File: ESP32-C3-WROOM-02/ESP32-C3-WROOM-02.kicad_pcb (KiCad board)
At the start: 2 copper layers, 25.4 x 38.1 mm, 22 parts, among them J1 ESP32-C3-DEVKITC-02-J1, J2 ESP32-C3-DEVKITC-02-J2, J3 ESPProg-UART, J4 USB2.0_C, SW1 SW_Push, SW2 SW_Push, U1 AMS1117-3.3, U2 ESP32-C3-WROOM-02

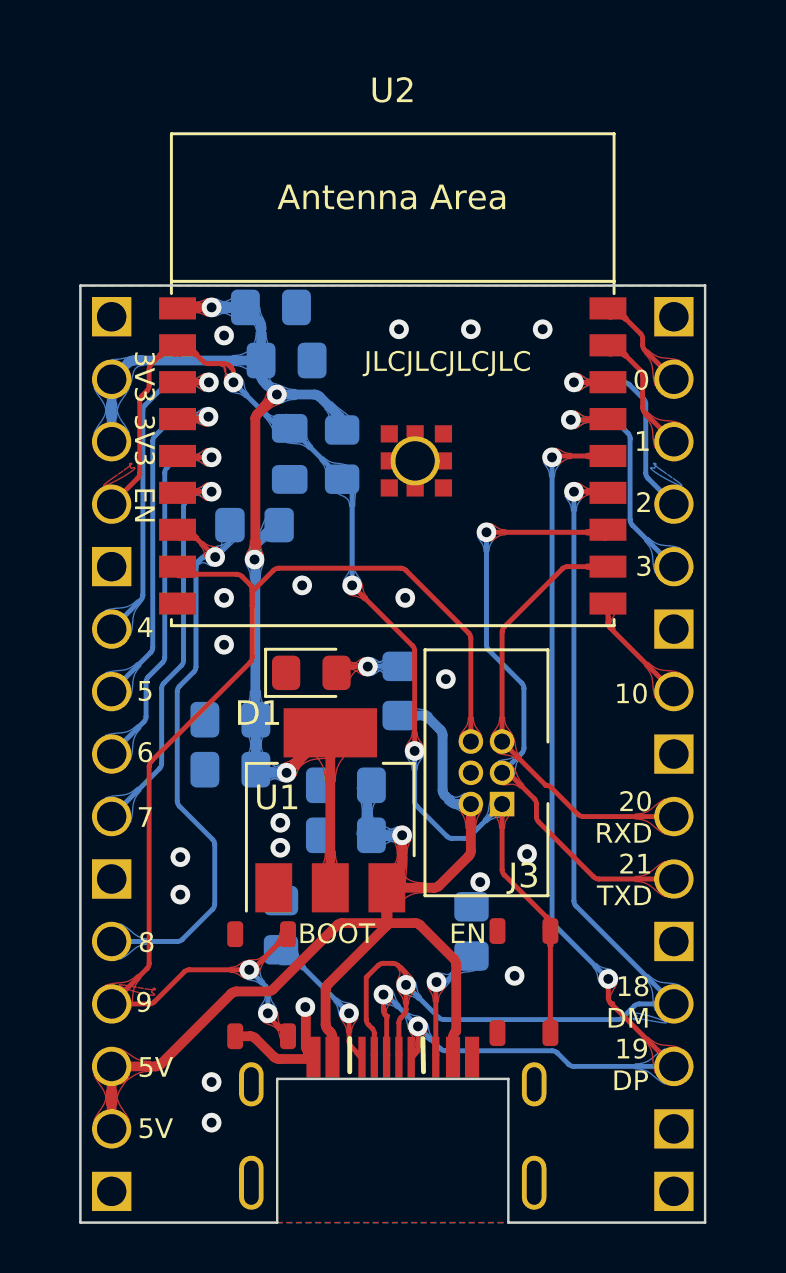
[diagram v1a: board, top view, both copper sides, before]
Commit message: esp3s-c3-devboard/v1.2.0
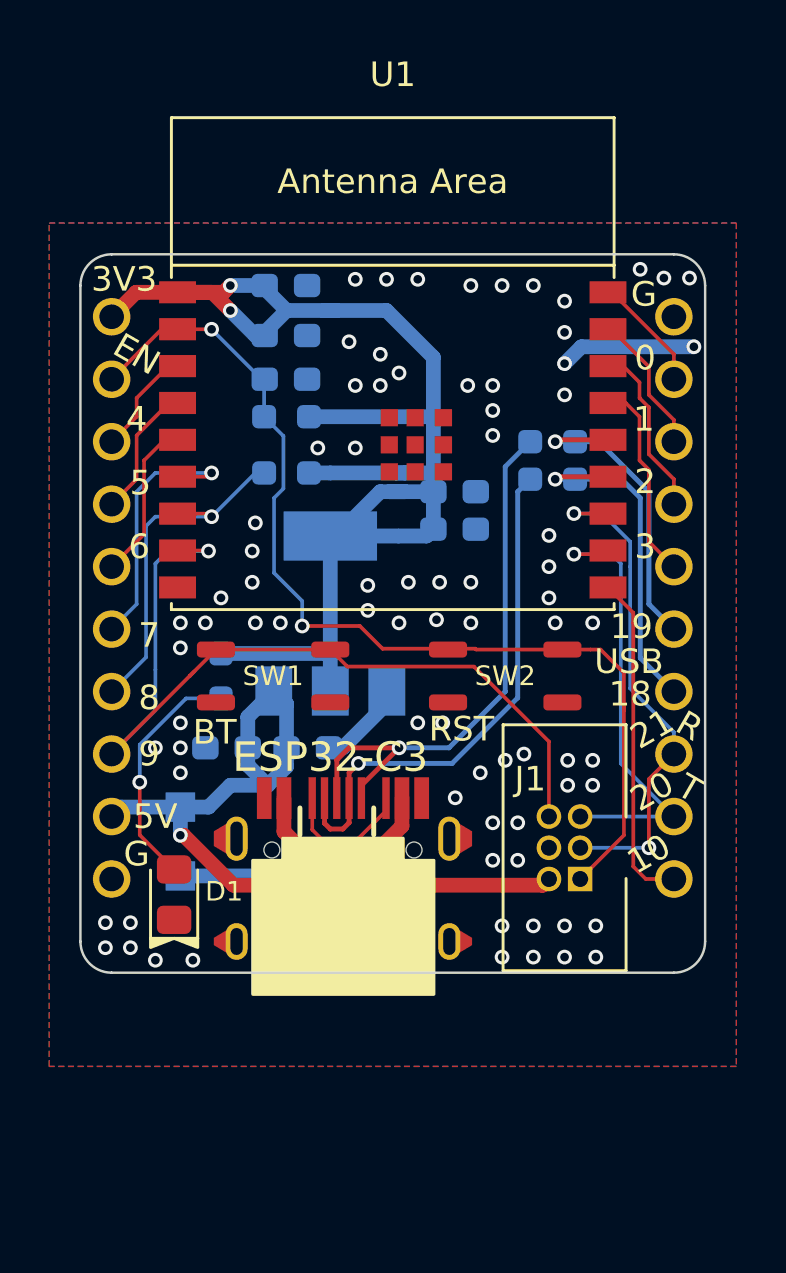
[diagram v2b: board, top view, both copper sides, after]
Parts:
- removed the J2 at (94.0, 48.3)
- removed J3: ESPProg-UART, esp32-dev-board:BoxPinHeader_2x03_P1.27mm_Vertical
- added CH1: Pin_10, 74th:PinOut_Pin_10, F.Cu at (72.4, 49.5)
- added CH2: Pin_10, 74th:PinOut_Pin_10, F.Cu at (95.2, 49.5)
- added D2: PMEG2010ER,115, 74th:Package_SOD123W, B.Cu at (75.2, 70.9)
- added R2: 10, 74th:Register_0603_1608, B.Cu at (90.3, 54.6)
- added R4: 10, 74th:Register_0603_1608, B.Cu at (90.3, 56.1)
- C1: renamed from C7; footprint esp32-dev-board:Capacitor_0805_2012 -> 74th:Capacitor_0603_1608
- C2: renamed from C6; footprint esp32-dev-board:Capacitor_0805_2012 -> 74th:Capacitor_0603_1608
- C3: renamed from C5; footprint esp32-dev-board:Capacitor_0805_2012 -> 74th:Capacitor_0603_1608
- C4: renamed from C3; footprint esp32-dev-board:Capacitor_0805_2012 -> 74th:Capacitor_0603_1608
- C5: renamed from C4; footprint esp32-dev-board:Capacitor_0805_2012 -> 74th:Capacitor_0603_1608
- C6: renamed from C1; footprint esp32-dev-board:Capacitor_0805_2012 -> 74th:Capacitor_0603_1608
- C7: renamed from C2; footprint esp32-dev-board:Capacitor_0805_2012 -> 74th:Capacitor_0603_1608
- D1: footprint LED_SMD:LED_0805_2012Metric_Pad1.15x1.40mm_HandSolder -> 74th:LED_0805_2012
- J1: value ESP32-C3-DEVKITC-02-J1 -> ESP-Prog-ProgramCOM_RECV; footprint esp32-dev-board:ESP32-C3-DEVKITC-J1 -> 74th:Connector_BoxPinHeader_2x03_P1.27mm
- J2: renamed from J4; footprint esp32-dev-board:USB-C-12-Pin-MidMount-ali-v4 -> 74th:Connector_USB-C-Receptacle_SMT_12-Pin_Simple
- R1: renamed from R2; footprint esp32-dev-board:Register_0805_2012 -> 74th:Register_0603_1608
- R3: renamed from R5; footprint esp32-dev-board:Register_0805_2012 -> 74th:Register_0603_1608
- R5: renamed from R1; footprint esp32-dev-board:Register_0805_2012 -> 74th:Register_0603_1608
- R6: renamed from R4; footprint esp32-dev-board:Register_0805_2012 -> 74th:Register_0603_1608
- R7: renamed from R3; footprint esp32-dev-board:Register_0805_2012 -> 74th:Register_0603_1608
- SW1: renamed from SW2; footprint esp32-dev-board:SKRPABE010 -> 74th:Switch_SKRPABE010
- SW2: renamed from SW1; footprint esp32-dev-board:SKRPABE010 -> 74th:Switch_SKRPABE010
- U1: renamed from U2; footprint esp32-dev-board:ESP32-C3-WROOM-02-handsolder -> PCM_Espressif:ESP32-C3-WROOM-02
- U2: renamed from U1; footprint Package_TO_SOT_SMD:SOT-223-3_TabPin2 -> 74th:Package_SOT-223-3; moved to B.Cu
- moved J1 30.2 mm to (90.8, 71.1), turned to 180 degrees
- moved C4 14.5 mm to (86.2, 56.6), turned to 0 degrees
- moved SW1 12.6 mm to (79.0, 64.1), turned to 180 degrees
- moved SW2 12.5 mm to (88.4, 64.1), turned to 180 degrees
- moved C5 11.9 mm to (86.2, 58.2), turned to 0 degrees
- moved D1 10.6 mm to (74.9, 73.0), turned to 90 degrees
- moved U2 8.00 mm to (81.3, 61.6)
- moved R5 7.38 mm to (76.8, 64.1), turned to -90 degrees
- moved J2 5.21 mm to (81.8, 74.8)
- moved C7 4.99 mm to (77.2, 67.1)
- moved C6 3.92 mm to (80.3, 67.1), turned to 0 degrees
- moved R6 3.84 mm to (83.3, 73.9), turned to -90 degrees
- moved C3 3.05 mm to (79.4, 52.1), turned to 0 degrees
- moved R1 2.71 mm to (79.5, 53.6), turned to 180 degrees
- moved R3 2.46 mm to (79.5, 55.9)
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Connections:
- C3 pad 1: EN -> /EN
- J1 pad 1: GND -> /EN
- J1 pad 2: +3V3 -> +5V
- J1 pad 3: +3V3 -> /IO21
- J1 pad 4: EN -> GND
- J1 pad 5: GND -> /IO20
- J1 pad 6: GPIO4 -> /IO9
- J2 pad 1: +5V -> Net-(D2-A)
- J2 pad 2: GPIO18 -> Net-(J4-D-)
- J2 pad 3: GPIO19 -> Net-(J4-D+)
- R1 pad 2: EN -> /EN
- R3 pad 2: GPIO8 -> /IO8
- R5 pad 1: +5V -> +3V3
- SW1 pad 2: GPIO9 -> /IO9
- SW2 pad 2: EN -> /EN
- U1 pad 10: GPIO10 -> /IO10
- U1 pad 11: GPIO20 -> /IO20
- U1 pad 12: GPIO21 -> /IO21
- U1 pad 13: GPIO18 -> /IO18
- U1 pad 14: GPIO19 -> /IO19
- U1 pad 15: GPIO3 -> /IO3
- U1 pad 16: GPIO2 -> /IO2
- U1 pad 17: GPIO1 -> /IO1
- U1 pad 18: GPIO0 -> /IO0
- U1 pad 2: EN -> /EN
- U1 pad 3: GPIO4 -> /IO4
- U1 pad 4: GPIO5 -> /IO5
- U1 pad 5: GPIO6 -> /IO6
- U1 pad 6: GPIO7 -> /IO7
- U1 pad 7: GPIO8 -> /IO8
- U1 pad 8: GPIO9 -> /IO9
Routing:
- net GPIO9: track 49.8 -> 0.00 mm, vias 2 -> 0
- net EN: track 46.0 -> 0.00 mm, vias 3 -> 0
- net GPIO19: track 46.0 -> 0.00 mm, vias 4 -> 0
- net GPIO18: track 44.4 -> 0.00 mm, vias 2 -> 0
- net /EN: track 0.00 -> 42.1 mm, vias 0 -> 2
- net /IO9: track 0.00 -> 36.5 mm, vias 0 -> 1
- net GPIO21: track 24.9 -> 0.00 mm, vias 1 -> 0
- net GPIO8: track 24.2 -> 0.00 mm, vias 1 -> 0
- net Net-(J4-D+): track 0.00 -> 22.8 mm, vias 0 -> 1
- net Net-(J4-D-): track 0.00 -> 21.5 mm, vias 0 -> 1
- net /IO21: track 0.00 -> 20.5 mm, vias 0 -> 2
- net /IO20: track 0.00 -> 18.5 mm, vias 0 -> 1
- net GPIO20: track 18.1 -> 0.00 mm
- net GPIO7: track 16.6 -> 0.00 mm, vias 1 -> 0
- net +5V: track 48.9 -> 32.9 mm
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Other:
- board size 25.4 x 38.1 mm -> 25.4 x 29.2 mm
- board text added: "18"
- board text added: "19"
- board text added: "20"
- board text added: "21"
- board text added: "74th-G011-1.2.0"
- board text added: "BT"
- board text added: "ESP32-C3"
- board text added: "G"
- board text added: "R"
- board text added: "RST"
- board text added: "T"
- board text added: "USB"
- board text added: "v1.2.0"
- board text removed: "18 DM"
- board text removed: "19 DP"
- board text removed: "20 RXD"
- board text removed: "21 TXD"
- board text removed: "ESPC3DevBoard"
- board text removed: "v1.1.0"
